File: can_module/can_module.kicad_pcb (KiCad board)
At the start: 2 copper layers, 14 parts, among them J201 RJ45, J202 Screw_Terminal_01x02, U201 PESD5V0L2UU_esd_diode, U202 MCP2551-I-SN, U203 MCP2515-xST, Y201 Crystal

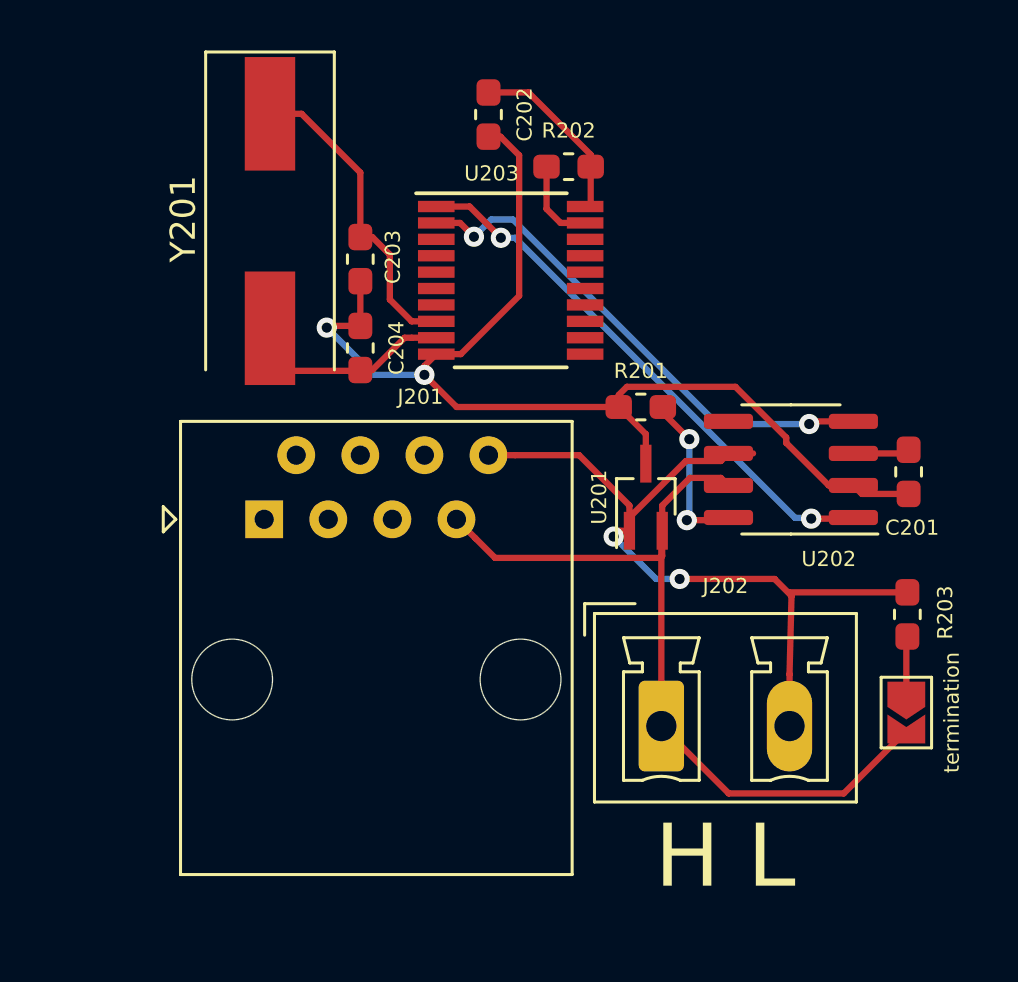
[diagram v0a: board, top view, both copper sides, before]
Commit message: controller v2 voor testvaart 1 mei
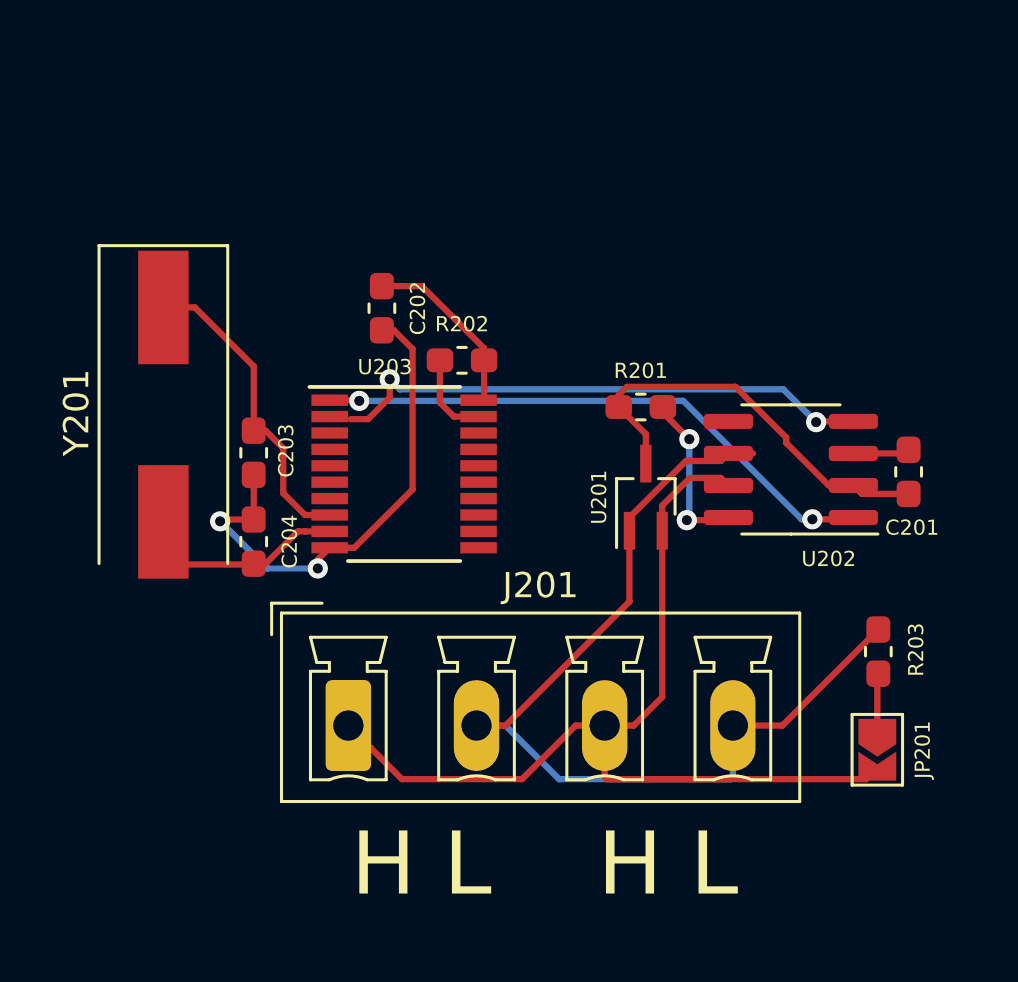
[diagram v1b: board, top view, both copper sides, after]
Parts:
- removed J202: Screw_Terminal_01x02, Connector_Phoenix_MC_HighVoltage:PhoenixContact_MCV_1,5_2-G-5.08_1x02_P5.08mm_Vertical
- J201: value RJ45 -> can; footprint Connector_RJ:RJ45_Amphenol_54602-x08_Horizontal -> Connector_Phoenix_MC_HighVoltage:PhoenixContact_MCV_1,5_4-G-5.08_1x04_P5.08mm_Vertical
- moved J201 8.83 mm to (107.7, 55.3)
- moved R202 8.76 mm to (112.2, 40.8)
- moved C203 8.76 mm to (103.9, 44.5)
- moved U203 8.76 mm to (109.9, 45.3)
- moved C202 8.76 mm to (109.0, 38.8)
- moved C204 8.76 mm to (103.9, 48.0)
- moved Y201 8.76 mm to (100.4, 43.0)
- moved JP201 1.87 mm to (128.7, 56.3)
- moved R203 1.87 mm to (128.7, 52.4)
- renumbered termination to JP201
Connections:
- J201 pad 1: Net-(J201-Pad1) -> /Sheet6074414D/can_h
- J201 pad 2: Net-(J201-Pad2) -> /Sheet6074414D/can_l
- J201 pad 3: Net-(J201-Pad3) -> /Sheet6074414D/can_h
- J201 pad 4: Net-(J201-Pad4) -> /Sheet6074414D/can_l
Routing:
- net GND: track 45.0 -> 36.8 mm
- net /Sheet6074414D/can_l: track 32.7 -> 37.8 mm, vias 2 -> 0
- net /Sheet6074414D/can_h: track 33.6 -> 38.5 mm
- net /Sheet6074414D/can_rx: track 20.4 -> 21.7 mm
- net /Sheet6074414D/can_tx: track 21.7 -> 22.7 mm
